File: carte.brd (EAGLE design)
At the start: 84 x 85 mm, 14 parts, among them J1 MIC127-140-A01

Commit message: régulation du contenu du répertoire GIT
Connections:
- net N$5 renamed P8
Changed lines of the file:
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@@
 <wire x1="24.285" y1="39.715" x2="25.75" y2="38.25" width="0.254" layer="1"/>
 </signal>
-<signal name="N$5">
+<signal name="P8">
 <contactref element="CAPTEUR_ULTRASON" pad="2"/>
 <contactref element="J1" pad="27"/>

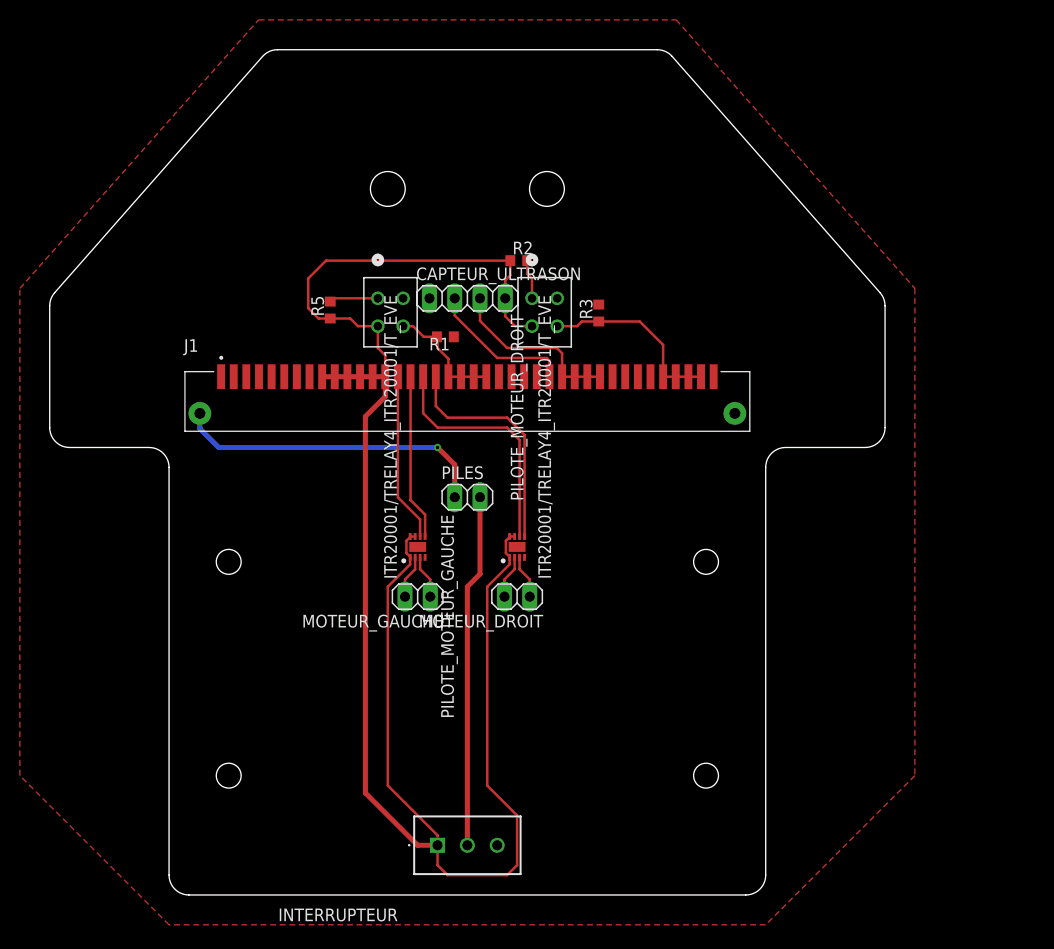
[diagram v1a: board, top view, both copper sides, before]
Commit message: régulation du contenu du répertoire GIT
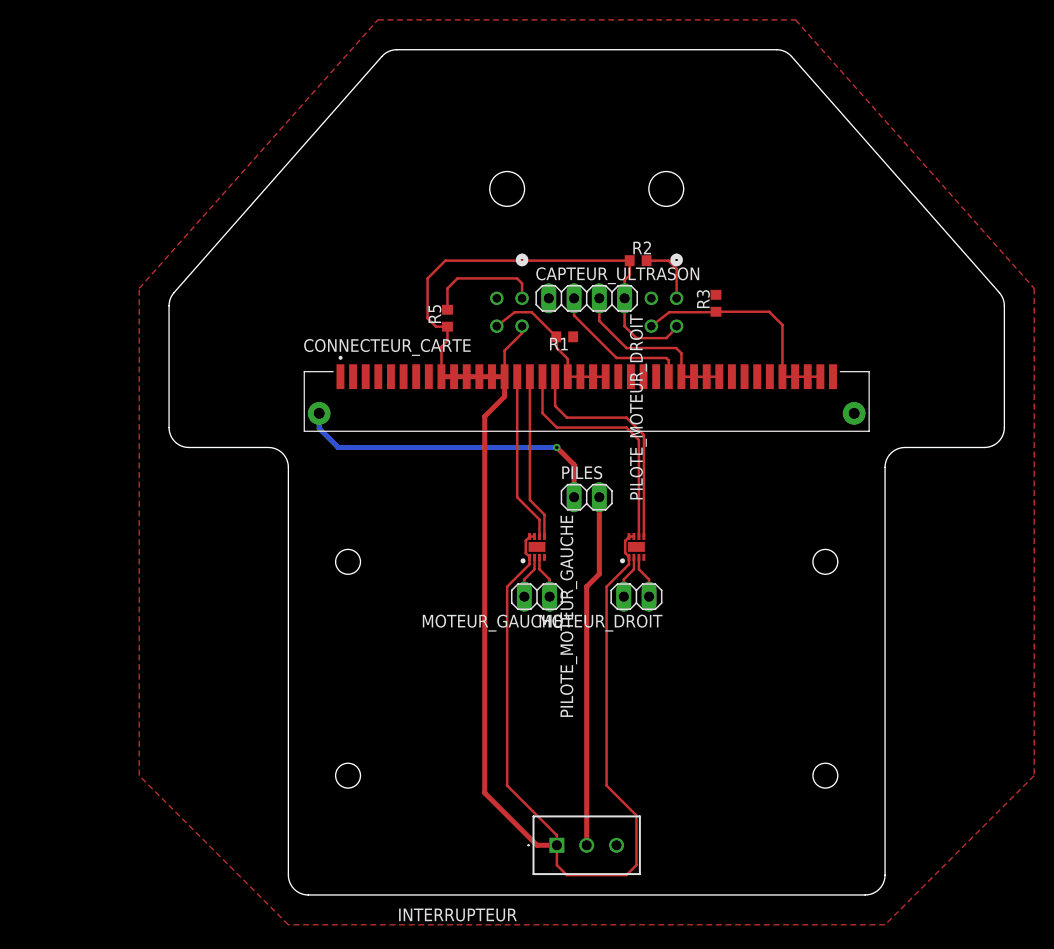
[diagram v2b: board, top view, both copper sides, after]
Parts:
- removed J1: MIC127-140-A01, MIC127-140-A01:DONGGUAN_MIC127-140-A01
- added CONNECTEUR_CARTE: MIC127-140-A01, MIC127-140-A01:DONGGUAN_MIC127-140-A01
- moved CAPTEUR_INFRAROUGE_DROIT 14.5 mm to (51.0, 60.0), flipped to the bottom
- moved CAPTEUR_INFRAROUGE_GAUCHE 14.5 mm to (35.5, 60.0), flipped to the bottom
- moved CAPTEUR_ULTRASON 12.0 mm to (42.0, 60.0)
- moved INTERRUPTEUR 12.0 mm to (39.0, 5.00)
- moved MOTEUR_DROIT 12.0 mm to (47.0, 30.0)
- moved MOTEUR_GAUCHE 12.0 mm to (37.0, 30.0)
- moved PILES 12.0 mm to (42.0, 40.0)
- moved PILOTE_MOTEUR_DROIT 12.0 mm to (47.0, 35.0)
- moved PILOTE_MOTEUR_GAUCHE 12.0 mm to (37.0, 35.0)
- moved R1 12.0 mm to (39.8, 56.1)
- moved R2 12.0 mm to (47.2, 63.8)
- moved R3 11.8 mm to (55.0, 59.5)
- moved R5 11.8 mm to (28.0, 58.0)
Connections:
- net 3V: now also CONNECTEUR_CARTE.10, CONNECTEUR_CARTE.11, CONNECTEUR_CARTE.12, CONNECTEUR_CARTE.13, CONNECTEUR_CARTE.14, CONNECTEUR_CARTE.9; no longer J1.10, J1.11, J1.12, J1.13, J1.14, J1.9
- net GND: now also CONNECTEUR_CARTE.1, CONNECTEUR_CARTE.2, CONNECTEUR_CARTE.3, CONNECTEUR_CARTE.4, CONNECTEUR_CARTE.5, CONNECTEUR_CARTE.6, CONNECTEUR_CARTE.S1, CONNECTEUR_CARTE.S2; no longer INTERRUPTEUR.3, J1.1, J1.2, J1.3, J1.4, J1.5, J1.6, J1.S1, J1.S2
- net P0: now also CONNECTEUR_CARTE.36, CONNECTEUR_CARTE.37, CONNECTEUR_CARTE.38, CONNECTEUR_CARTE.39; no longer J1.36, J1.37, J1.38, J1.39
- net P1: now also CONNECTEUR_CARTE.28, CONNECTEUR_CARTE.29, CONNECTEUR_CARTE.30, CONNECTEUR_CARTE.31; no longer J1.28, J1.29, J1.30, J1.31
- net P13: now also CONNECTEUR_CARTE.18; no longer J1.18
- net P14: now also CONNECTEUR_CARTE.17; no longer J1.17
- net P15: now also CONNECTEUR_CARTE.16; no longer J1.16
- net P16: now also CONNECTEUR_CARTE.15; no longer J1.15
- net P2: now also CONNECTEUR_CARTE.19, CONNECTEUR_CARTE.20, CONNECTEUR_CARTE.21, CONNECTEUR_CARTE.22; no longer J1.19, J1.20, J1.21, J1.22
- net P8: now also CONNECTEUR_CARTE.27; no longer J1.27
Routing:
- net N$6: track 4.93 -> 11.8 mm
- net 3V: track 186.3 -> 191.8 mm
- net P0: track 18.8 -> 23.2 mm
- net P2: track 12.1 -> 15.8 mm
- net N$11: track 3.99 -> 6.32 mm
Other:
- board text removed: "/Users/pierr_paul/Downloads/lien URL GitHub.bmp"
